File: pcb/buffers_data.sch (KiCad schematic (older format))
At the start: 8 parts, among them U1 74LVCH162245A, U2 74LVCH162245A

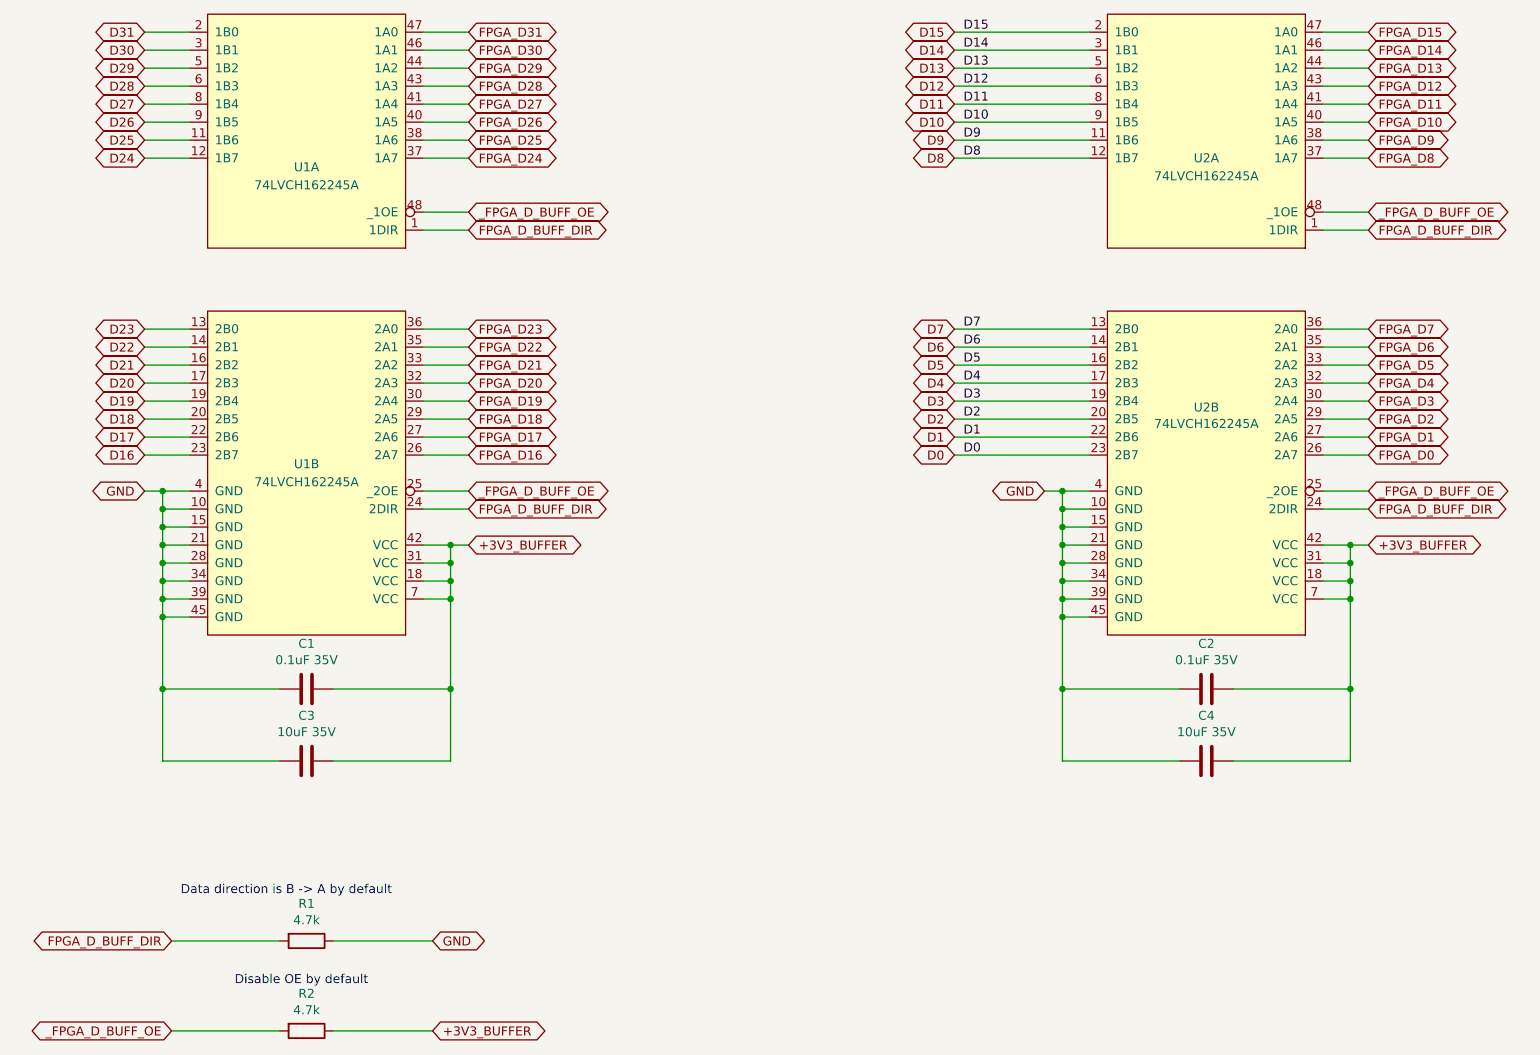
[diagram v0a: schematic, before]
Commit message: working on pcb 2
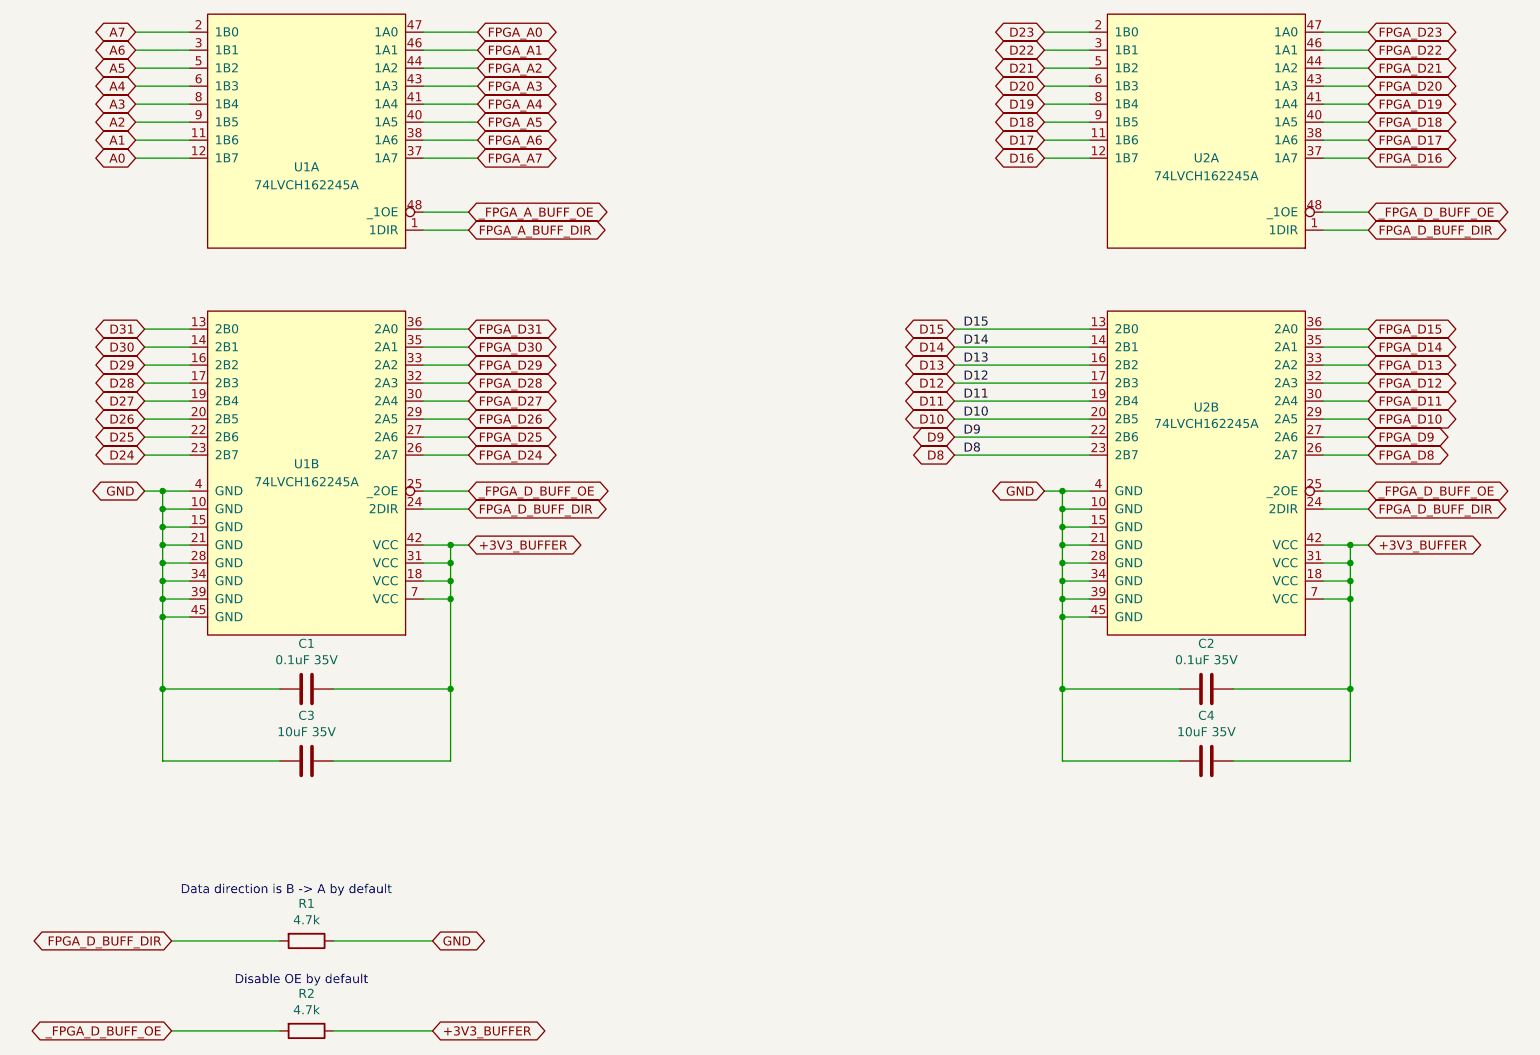
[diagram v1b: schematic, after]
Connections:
- net D0 is gone; now on net D8: U2.23 (2B7)
- net D1 is gone; now on net D9: U2.22 (2B6)
- net D2 is gone; now on net D10: U2.20 (2B5)
- net D3 is gone; now on net D11: U2.19 (2B4)
- net D4 is gone; now on net D12: U2.17 (2B3)
- net D5 is gone; now on net D13: U2.16 (2B2)
- net D6 is gone; now on net D14: U2.14 (2B1)
- net D7 is gone; now on net D15: U2.13 (2B0)
- net FPGA_D0 is gone; now on net FPGA_D8: U2.26 (2A7)
- net FPGA_D1 is gone; now on net FPGA_D9: U2.27 (2A6)
- net FPGA_D2 is gone; now on net FPGA_D10: U2.29 (2A5)
- net FPGA_D3 is gone; now on net FPGA_D11: U2.30 (2A4)
- net FPGA_D4 is gone; now on net FPGA_D12: U2.32 (2A3)
- net FPGA_D5 is gone; now on net FPGA_D13: U2.33 (2A2)
- net FPGA_D6 is gone; now on net FPGA_D14: U2.35 (2A1)
- net FPGA_D7 is gone; now on net FPGA_D15: U2.36 (2A0)
- net D10: no longer U2.9 (1B5)
- net D11: no longer U2.8 (1B4)
- net D12: no longer U2.6 (1B3)
- net D13: no longer U2.5 (1B2)
- net D14: no longer U2.3 (1B1)
- net D15: no longer U2.2 (1B0)
- net D16: now also U2.12 (1B7); no longer U1.23 (2B7)
- net D17: now also U2.11 (1B6); no longer U1.22 (2B6)
- net D18: now also U2.9 (1B5); no longer U1.20 (2B5)
- net D19: now also U2.8 (1B4); no longer U1.19 (2B4)
- net D20: now also U2.6 (1B3); no longer U1.17 (2B3)
- net D21: now also U2.5 (1B2); no longer U1.16 (2B2)
- net D22: now also U2.3 (1B1); no longer U1.14 (2B1)
- net D23: now also U2.2 (1B0); no longer U1.13 (2B0)
- net D24: now also U1.23 (2B7); no longer U1.12 (1B7)
- net D25: now also U1.22 (2B6); no longer U1.11 (1B6)
- net D26: now also U1.20 (2B5); no longer U1.9 (1B5)
- net D27: now also U1.19 (2B4); no longer U1.8 (1B4)
- net D28: now also U1.17 (2B3); no longer U1.6 (1B3)
- net D29: now also U1.16 (2B2); no longer U1.5 (1B2)
- net D30: now also U1.14 (2B1); no longer U1.3 (1B1)
- net D31: now also U1.13 (2B0); no longer U1.2 (1B0)
- net D8: no longer U2.12 (1B7)
- net D9: no longer U2.11 (1B6)
- net FPGA_D10: no longer U2.40 (1A5)
- net FPGA_D11: no longer U2.41 (1A4)
- net FPGA_D12: no longer U2.43 (1A3)
- net FPGA_D13: no longer U2.44 (1A2)
- net FPGA_D14: no longer U2.46 (1A1)
- net FPGA_D15: no longer U2.47 (1A0)
- net FPGA_D16: now also U2.37 (1A7); no longer U1.26 (2A7)
- net FPGA_D17: now also U2.38 (1A6); no longer U1.27 (2A6)
- net FPGA_D18: now also U2.40 (1A5); no longer U1.29 (2A5)
- net FPGA_D19: now also U2.41 (1A4); no longer U1.30 (2A4)
- net FPGA_D20: now also U2.43 (1A3); no longer U1.32 (2A3)
- net FPGA_D21: now also U2.44 (1A2); no longer U1.33 (2A2)
- net FPGA_D22: now also U2.46 (1A1); no longer U1.35 (2A1)
- net FPGA_D23: now also U2.47 (1A0); no longer U1.36 (2A0)
- net FPGA_D24: now also U1.26 (2A7); no longer U1.37 (1A7)
- net FPGA_D25: now also U1.27 (2A6); no longer U1.38 (1A6)
- net FPGA_D26: now also U1.29 (2A5); no longer U1.40 (1A5)
- net FPGA_D27: now also U1.30 (2A4); no longer U1.41 (1A4)
- net FPGA_D28: now also U1.32 (2A3); no longer U1.43 (1A3)
- net FPGA_D29: now also U1.33 (2A2); no longer U1.44 (1A2)
- net FPGA_D30: now also U1.35 (2A1); no longer U1.46 (1A1)
- net FPGA_D31: now also U1.36 (2A0); no longer U1.47 (1A0)
- net FPGA_D8: no longer U2.37 (1A7)
- net FPGA_D9: no longer U2.38 (1A6)
- net FPGA_D_BUFF_DIR: no longer U1.1 (1DIR)
- net _FPGA_D_BUFF_OE: no longer U1.48 (_1OE)
- new net A0: U1.12 (1B7)
- new net A1: U1.11 (1B6)
- new net A2: U1.9 (1B5)
- new net A3: U1.8 (1B4)
- new net A4: U1.6 (1B3)
- new net A5: U1.5 (1B2)
- new net A6: U1.3 (1B1)
- new net A7: U1.2 (1B0)
- new net FPGA_A0: U1.47 (1A0)
- new net FPGA_A1: U1.46 (1A1)
- new net FPGA_A2: U1.44 (1A2)
- new net FPGA_A3: U1.43 (1A3)
- new net FPGA_A4: U1.41 (1A4)
- new net FPGA_A5: U1.40 (1A5)
- new net FPGA_A6: U1.38 (1A6)
- new net FPGA_A7: U1.37 (1A7)
- new net FPGA_A_BUFF_DIR: U1.1 (1DIR)
- new net _FPGA_A_BUFF_OE: U1.48 (_1OE)
